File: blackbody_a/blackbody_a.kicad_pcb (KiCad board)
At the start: 2 copper layers, 48.9 x 38.5 mm, 65 parts, among them IC1 LM76202QPWPRQ1, IC2 TPS562231DRLR, SW4 SW_SPDT, SW5 SW_Push, SW6 Reset, U1 LTC4311CSC6-TRPBF, U2 TCAN337DCNR, U3 STM32L431CBTx, Y1 8M

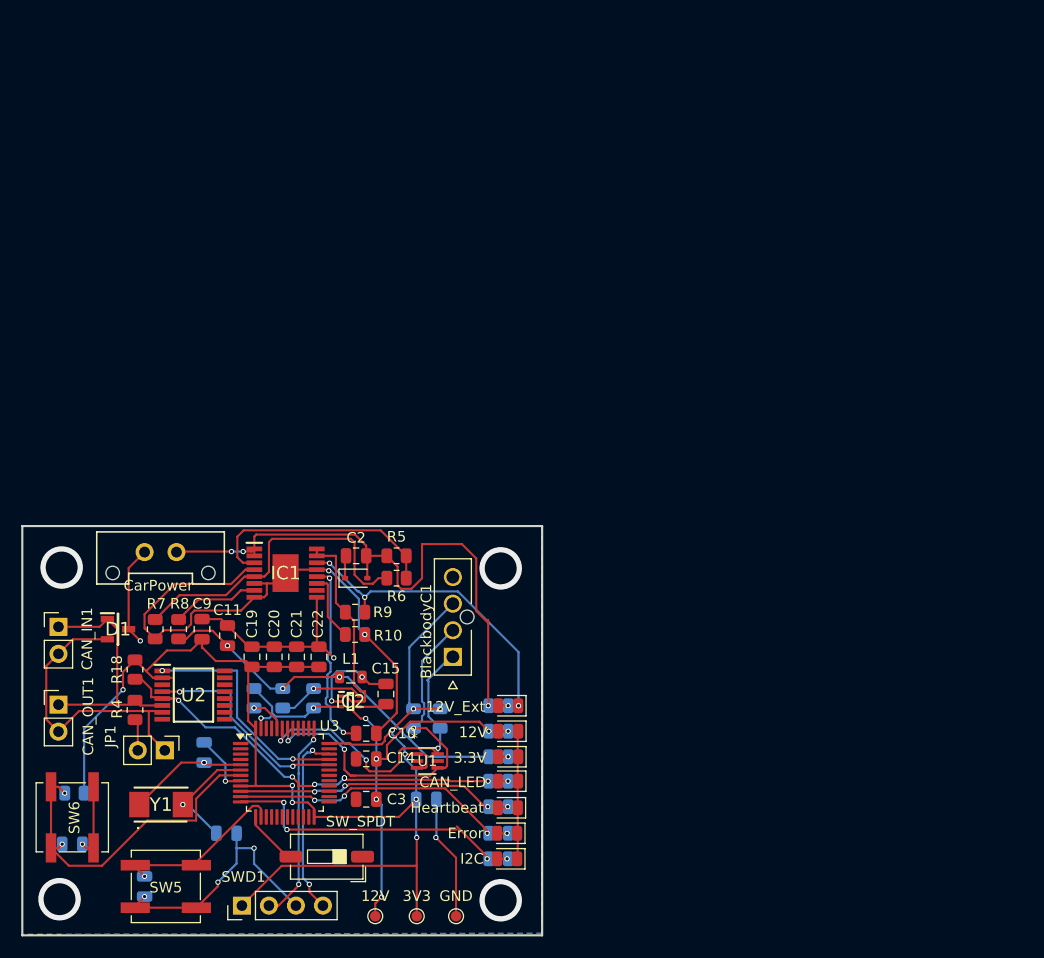
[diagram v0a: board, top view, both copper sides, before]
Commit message: layout edits
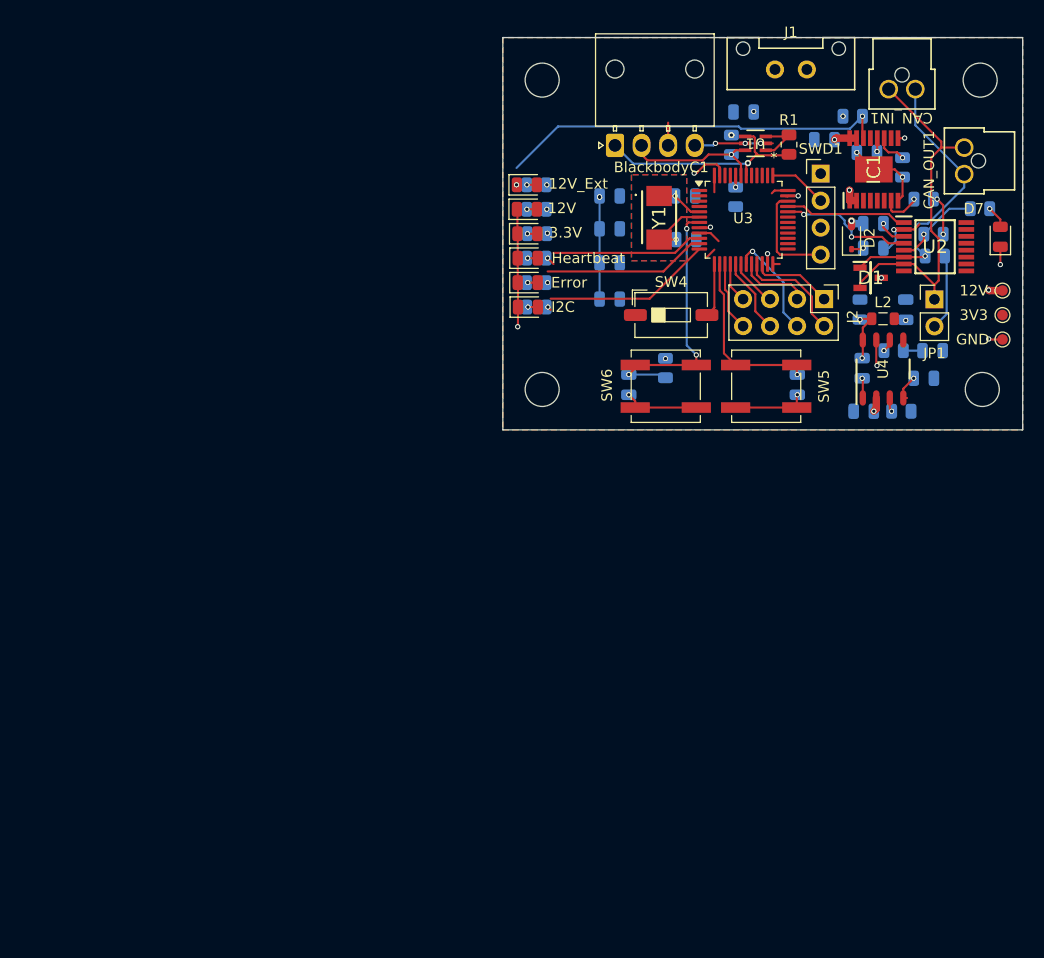
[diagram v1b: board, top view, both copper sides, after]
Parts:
- removed C11: 47uF, Capacitor_SMD:C_0805_2012Metric
- removed C14: 10uF, Capacitor_SMD:C_0805_2012Metric
- removed C15: 0.1uF, Capacitor_SMD:C_0805_2012Metric
- removed CarPower: CarPowerConnector, UTSVT_Connectors:Molex_MicroFit3.0_1x2xP3.00mm_PolarizingPeg_Vertical
- removed IC2: TPS562231DRLR, blackbody_a:TPS562231DRLR
- removed L1: 3.3uH, Inductor_SMD:L_0805_2012Metric
- removed R11: 45.3k, Resistor_SMD:R_0805_2012Metric
- removed R12: 10k, Resistor_SMD:R_0805_2012Metric
- removed R6: 200, Resistor_SMD:R_0805_2012Metric
- removed R7: 1k, Resistor_SMD:R_0805_2012Metric
- added C16: 10uF, Capacitor_SMD:C_0805_2012Metric, B.Cu at (148.1, 115.6)
- added C17: 0.1uF, Capacitor_SMD:C_0805_2012Metric, B.Cu at (147.9, 111.5)
- added C18: 10nF, Capacitor_SMD:C_0805_2012Metric, B.Cu at (153.7, 112.5)
- added C25: 4.7nF, Capacitor_SMD:C_0805_2012Metric, B.Cu at (154.5, 109.9)
- added C4: 33uF, Capacitor_SMD:C_0805_2012Metric, B.Cu at (152.0, 106.0)
- added D6: D, Diode_SMD:D_0805_2012Metric, B.Cu at (147.7, 106.0)
- added H1: MountingHole, MountingHole:MountingHole_3.2mm_M3, F.Cu at (117.8, 113.5)
- added H2: MountingHole, MountingHole:MountingHole_3.2mm_M3, F.Cu at (159.0, 84.4)
- added H3: MountingHole, MountingHole:MountingHole_3.2mm_M3, F.Cu at (159.2, 113.5)
- added H4: MountingHole, MountingHole:MountingHole_3.2mm_M3, F.Cu at (117.8, 84.4)
- added J1: CarPowerConnector, UTSVT_Connectors:Molex_MicroFit3.0_1x2xP3.00mm_PolarizingPeg_Vertical, F.Cu at (139.7, 83.4)
- added J2: Conn_02x04_Counter_Clockwise, Connector_PinHeader_2.54mm:PinHeader_2x04_P2.54mm_Vertical, F.Cu at (144.3, 105.0)
- added L2: 13.3uH, Inductor_SMD:L_0805_2012Metric, F.Cu at (149.9, 106.9)
- added Rosc1: 85.5k, Resistor_SMD:R_0805_2012Metric, B.Cu at (151.6, 115.6)
- added U4: TPS5403DR, blackbodies:D0008A_N, F.Cu at (149.9, 111.6)
- BlackbodyC1: footprint blackbodies:MOLEX_1053091104 -> Connector_Molex:Molex_Nano-Fit_105313-xx04_1x04_P2.50mm_Horizontal
- C10, C19, C2, C20, C21, C22, C3, C9, R18, R4, R8, R9: moved to B.Cu
- CAN_IN1, CAN_OUT1: footprint Connector_PinHeader_2.54mm:PinHeader_1x02_P2.54mm_Vertical -> blackbodies:CONN_SD-105309-100_02_MOL
- R1: moved to F.Cu
- R10: value 10K -> 20K; moved to B.Cu
- R5: value 10k -> 12k; moved to B.Cu
- moved CAN_OUT1 98.7 mm to (157.5, 93.3), turned to 90 degrees
- moved CAN_IN1 95.2 mm to (152.9, 85.3), turned to 180 degrees
- moved SWD1 87.8 mm to (144.0, 93.2), turned to 0 degrees
- moved R4 86.5 mm to (154.7, 101.0), turned to 0 degrees
- moved R18 85.5 mm to (154.6, 98.9), turned to 180 degrees
- moved JP1 83.9 mm to (154.7, 105.1), turned to 0 degrees
- moved TP1 83.3 mm to (161.1, 104.2)
- moved U2 81.5 mm to (154.8, 100.1)
- moved R8 80.9 mm to (153.7, 95.6), turned to 180 degrees
- moved TP4 79.0 mm to (161.1, 106.5)
- moved D1 78.1 mm to (148.7, 103.0)
- moved C23 77.4 mm to (141.8, 113.1)
- moved C3 75.6 mm to (144.3, 90.0)
- moved TP5 74.7 mm to (161.1, 108.8)
- moved SW5 73.5 mm to (138.9, 113.2)
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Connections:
- BlackbodyC1 pad 1: /SDA -> /SCL
- BlackbodyC1 pad 2: /SCL -> /SDA
- BlackbodyC1 pad 3: +3V3 -> +3.3V
- C1 pad 2: +3V3 -> +3.3V
- C19 pad 1: +3V3 -> +3.3V
- C20 pad 1: +3V3 -> +3.3V
- C21 pad 1: +3V3 -> +3.3V
- C22 pad 1: +3V3 -> +3.3V
- C9 pad 1: +3V3 -> +3.3V
- IC1 pad 13: /power_dist/RTN -> unconnected-(IC1-NC_2-Pad13)
- IC1 pad 4: /power_dist/RTN -> unconnected-(IC1-NC_1-Pad4)
- IC1 pad 6: /power_dist/RTN -> /power_dist/MODE
- R1 pad 1: +3V3 -> +3.3V
- R18 pad 1: +3V3 -> +3.3V
- R2 pad 1: +3V3 -> +3.3V
- R23 pad 1: +3V3 -> +3.3V
- R5 pad 1: /12V_Ext -> Net-(U4-COMP)
- R5 pad 2: /power_dist/UVLO -> Net-(C25-Pad2)
- SWD1 pad 1: +3V3 -> +3.3V
- U1 pad 1: +3V3 -> +3.3V
- U1 pad 3: +3V3 -> +3.3V
- U2 pad 2: +3V3 -> +3.3V
- U3 pad 15: unconnected-(U3-PA5-Pad15) -> /15
- U3 pad 16: unconnected-(U3-PA6-Pad16) -> /16
- U3 pad 17: unconnected-(U3-PA7-Pad17) -> /17
- U3 pad 18: unconnected-(U3-PB0-Pad18) -> /18
- U3 pad 19: unconnected-(U3-PB1-Pad19) -> /19
- U3 pad 20: unconnected-(U3-PB2-Pad20) -> /20
- U3 pad 21: unconnected-(U3-PB10-Pad21) -> /21
- U3 pad 22: unconnected-(U3-PB11-Pad22) -> /22
- U3 pad 24: +3V3 -> +3.3V
- U3 pad 36: +3V3 -> +3.3V
- U3 pad 48: +3V3 -> +3.3V
- U3 pad 9: +3V3 -> +3.3V
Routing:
- net +3V3: track 134.4 -> 0.00 mm, vias 9 -> 0
- net GND: track 103.9 -> 48.9 mm, vias 10 -> 17
- net /12V_Ext: track 54.9 -> 3.44 mm
- net +12V: track 55.5 -> 4.73 mm
- net /power_dist/RTN: track 55.1 -> 7.65 mm
- net /can_comm/Fault: track 39.6 -> 8.20 mm, vias 6 -> 1
- net /power_dist/OVP: track 30.3 -> 0.00 mm
- net /power_dist/UVLO: track 23.0 -> 0.00 mm
- net /SDA: track 31.1 -> 13.6 mm, vias 3 -> 1
- net Net-(IC1-DVDT): track 18.2 -> 1.27 mm, vias 2 -> 1
- net /SCL: track 36.0 -> 21.8 mm, vias 3 -> 1
- net /SWCLK: track 19.0 -> 5.48 mm, vias 2 -> 0
- net /I2C: track 27.0 -> 16.3 mm, vias 3 -> 1
- net /Error: track 25.8 -> 15.4 mm, vias 3 -> 1
- net /19: track 0.00 -> 10.3 mm, vias 0 -> 1
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- added copper zone on B.Cu, net (none)
- added copper zone on F.Cu, net (none)
- added copper zone on In1.Cu, net (none)
- added copper zone on In2.Cu, net (none)
- added copper zone on In1.Cu, net +12V
- added copper zone on F.Cu, net +3.3V
- added copper zone on In2.Cu, net /12V_Ext
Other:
- board size 48.9 x 38.5 mm -> 48.9 x 36.9 mm
- copper layers 2 -> 4

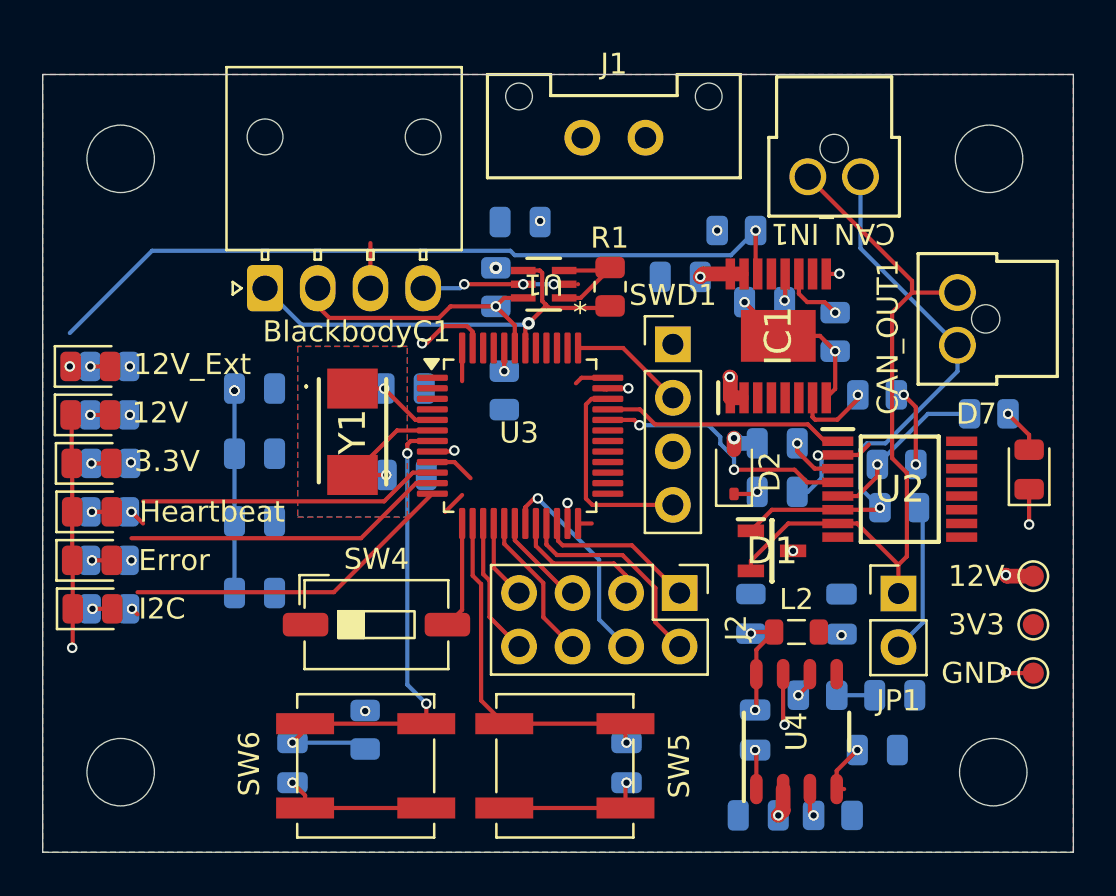
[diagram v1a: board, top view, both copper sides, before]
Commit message: layout updates
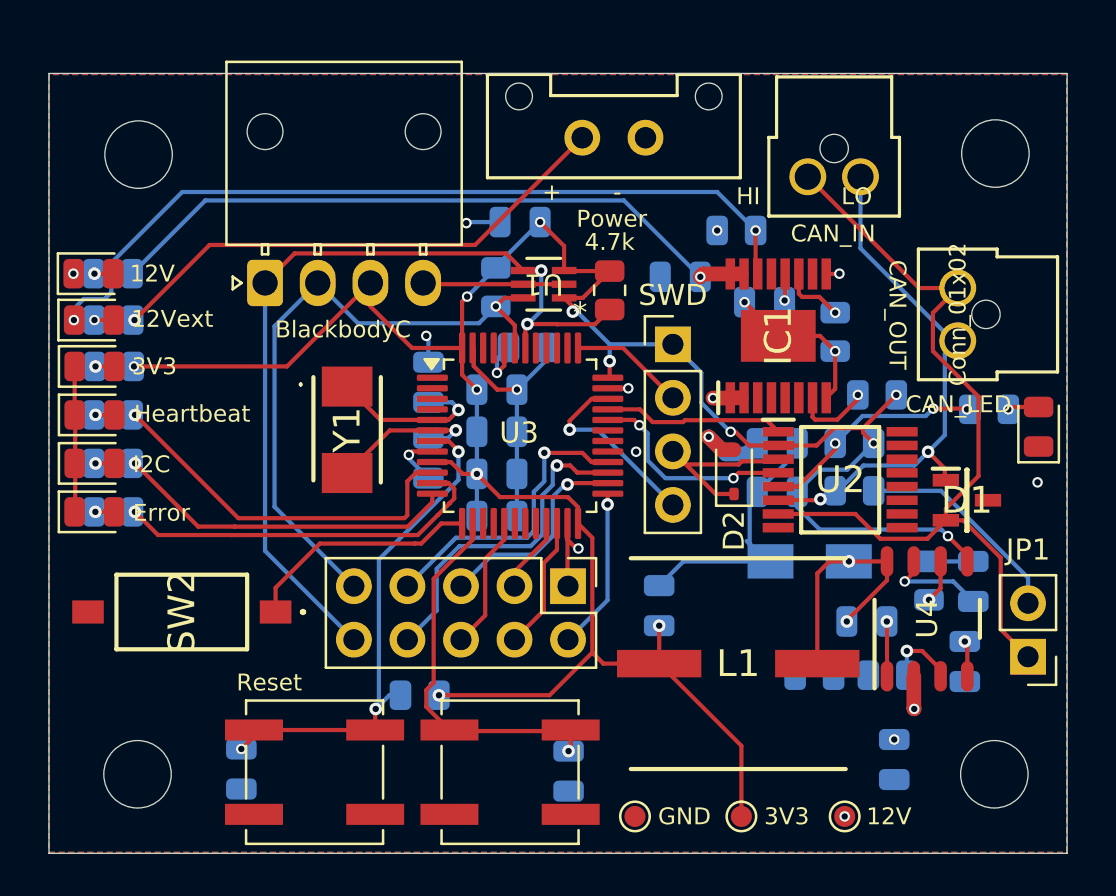
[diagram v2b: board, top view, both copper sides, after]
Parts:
- removed D11: I2C, LED_SMD:LED_0805_2012Metric
- removed D12: Heartbeat, LED_SMD:LED_0805_2012Metric
- removed D3: 12V, LED_SMD:LED_0805_2012Metric
- removed D4: 3.3V, LED_SMD:LED_0805_2012Metric
- removed D5: 12V_Ext, LED_SMD:LED_0805_2012Metric
- removed D8: Error, LED_SMD:LED_0805_2012Metric
- removed J2: Conn_02x04_Counter_Clockwise, Connector_PinHeader_2.54mm:PinHeader_2x04_P2.54mm_Vertical
- removed L2: 13.3uH, Inductor_SMD:L_0805_2012Metric
- removed SW4: SW_SPDT, Button_Switch_SMD:SW_DIP_SPSTx01_Slide_6.7x4.1mm_W6.73mm_P2.54mm_LowProfile_JPin
- removed TP1: 12V, TestPoint:TestPoint_Pad_D1.0mm
- removed TP4: 3V3, TestPoint:TestPoint_Pad_D1.0mm
- removed TP5: GND, TestPoint:TestPoint_Pad_D1.0mm
- added 12V: 12V, LED_SMD:LED_0805_2012Metric, F.Cu at (116.5, 89.9)
- added 12V: TestPoint, TestPoint:TestPoint_Pad_D1.0mm, F.Cu at (152.2, 115.7)
- added 12Vext: 12V, LED_SMD:LED_0805_2012Metric, F.Cu at (116.5, 92.1)
- added 3V3: TestPoint, TestPoint:TestPoint_Pad_D1.0mm, F.Cu at (147.2, 115.7)
- added 3V3: 3.3V, LED_SMD:LED_0805_2012Metric, F.Cu at (116.6, 94.3)
- added Error: Error, LED_SMD:LED_0805_2012Metric, F.Cu at (116.5, 101.2)
- added G***: LOGO, LOGO, B.Cu at (128.4, 86.5)
- added G***: LOGO, LOGO, B.Cu at (119.7, 105.9)
- added GND: TestPoint, TestPoint:TestPoint_Pad_D1.0mm, F.Cu at (142.2, 115.7)
- added Heartbeat: Heartbeat, LED_SMD:LED_0805_2012Metric, F.Cu at (116.6, 96.6)
- added I2C: I2C, LED_SMD:LED_0805_2012Metric, F.Cu at (116.6, 98.9)
- added J3: Conn_02x05_Counter_Clockwise, Connector_PinHeader_2.54mm:PinHeader_2x05_P2.54mm_Vertical, F.Cu at (139.0, 104.7)
- added L1: MSS1038-153MLC, blackbody_a:INDPM102100X400N, F.Cu at (147.1, 108.4)
- added Rosc2: 1k, Resistor_SMD:R_0805_2012Metric, B.Cu at (150.7, 109.0)
- added SW2: SW_DIP_x01, blackbodies:DS04254101BKSMT, F.Cu at (120.7, 106.0)
- C18: value 10nF -> 15nF
- C25: value 4.7nF -> 1nF
- C4: value 33uF -> 22uF
- D6: footprint Diode_SMD:D_0805_2012Metric -> blackbodies:SMA_DIO
- R18: value 2.2k -> 10k
- R5: value 12k -> 10k
- Rosc1: value 85.5k -> 84.5k
- moved H3 50.0 mm to (118.7, 84.2)
- moved H1 41.5 mm to (159.2, 113.7)
- moved H4 29.2 mm to (118.6, 113.7)
- moved C19 12.1 mm to (135.7, 101.4)
- moved C20 11.7 mm to (135.7, 99.4)
- moved C21 11.5 mm to (135.7, 97.4)
- moved C22 11.5 mm to (135.7, 95.4)
- moved D1 9.56 mm to (157.9, 100.7)
- moved C4 8.66 mm to (143.3, 105.7)
- moved U4 8.19 mm to (156.1, 106.3)
- moved R5 7.58 mm to (156.2, 104.5), turned to 90 degrees
- moved C17 7.39 mm to (153.2, 106.4), turned to 180 degrees
- moved Rosc1 7.14 mm to (154.2, 109.0), turned to 180 degrees
- moved C16 6.97 mm to (154.5, 113.0), turned to 90 degrees
- moved R21 6.90 mm to (117.4, 98.9)
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- renumbered BlackbodyC1 to BlackbodyC, D7 to CAN_Err, CAN_IN1 to CAN_IN, CAN_OUT1 to CAN_OUT, J1 to Power, SW6 to Reset, SWD1 to SWD
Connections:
- Rosc1 pad 2: GND -> Net-(Rosc1-Pad2)
- U3 pad 15: /15 -> unconnected-(U3-PA5-Pad15)
- U3 pad 16: /16 -> unconnected-(U3-PA6-Pad16)
- U3 pad 18: /18 -> unconnected-(U3-PB0-Pad18)
- U3 pad 19: /19 -> unconnected-(U3-PB1-Pad19)
- U3 pad 20: /20 -> unconnected-(U3-PB2-Pad20)
- U3 pad 21: /21 -> /UART_RX
- U3 pad 22: /22 -> /UART_TX
- U3 pad 25: unconnected-(U3-PB12-Pad25) -> /SPI_SS
- U3 pad 26: unconnected-(U3-PB13-Pad26) -> /SPI_SCK
- U3 pad 27: unconnected-(U3-PB14-Pad27) -> /SPI_MISO
- U3 pad 28: unconnected-(U3-PB15-Pad28) -> /SPI_MOSI
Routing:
- net +3.3V: track 33.3 -> 117.7 mm, vias 10 -> 13
- net /12V_Ext: track 3.44 -> 32.4 mm
- net +12V: track 4.73 -> 33.5 mm
- net /SCL: track 21.8 -> 41.1 mm, vias 1 -> 2
- net GND: track 48.9 -> 67.0 mm, vias 17 -> 11
- net /SDA: track 13.6 -> 30.2 mm
- net /SPI_MISO: track 0.00 -> 15.8 mm, vias 0 -> 1
- net /SPI_MOSI: track 0.00 -> 14.2 mm, vias 0 -> 1
- net /19: track 10.3 -> 0.00 mm, vias 1 -> 0
- net /21: track 10.3 -> 0.00 mm
- net /SPI_SCK: track 0.00 -> 10.1 mm, vias 0 -> 1
- net /SPI_SS: track 0.00 -> 7.71 mm, vias 0 -> 1
- net /22: track 7.67 -> 0.00 mm
- net /20: track 6.75 -> 0.00 mm
- net /15: track 6.54 -> 0.00 mm
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- added copper zone on F.Cu, net GND
- added copper zone on In1.Cu, net GND
- added copper zone on In2.Cu, net GND
- removed copper zone on B.Cu, net (none)
- removed copper zone on F.Cu, net (none)
- removed copper zone on In1.Cu, net (none)
- removed copper zone on In2.Cu, net (none)
- removed copper zone on F.Cu, net +3.3V
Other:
- board size 48.9 x 36.9 mm -> 48.3 x 37 mm
- board text added: "+ -"
- board text added: "BlackbodyA v1.0 Tanya Lertpradist Spring 2025"
- board text added: "HI LO"
- board text added: "MISO"
- board text added: "MOSI"
- board text added: "PA7"
- board text added: "RX"
- board text added: "SCK"
- board text added: "SCL"
- board text added: "SDA"
- board text added: "SS"
- board text added: "TX"
